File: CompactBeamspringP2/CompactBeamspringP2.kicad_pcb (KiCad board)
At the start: 2 copper layers, 162.3 x 33.2 mm, 54 parts, among them J1 BEAMSPRING CONNECTOR, J3 EXPANSION HEADER, U1 MCP4921-E, U2 LM339A, U3 74AHC595, U4 74AHC595, U5 ProMicro, U7 74AHC595

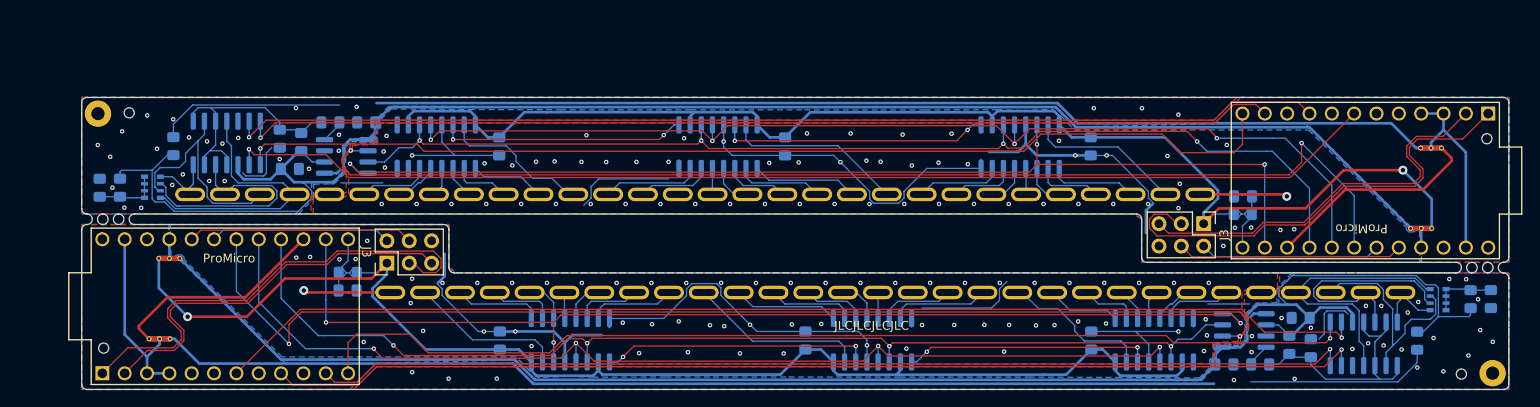
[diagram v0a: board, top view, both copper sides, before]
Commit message: More mods
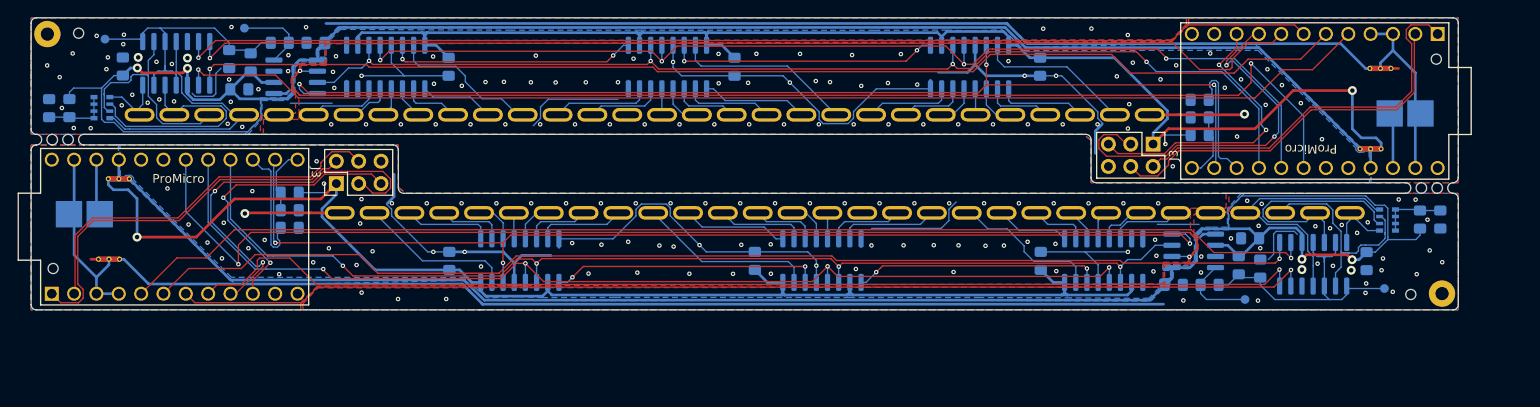
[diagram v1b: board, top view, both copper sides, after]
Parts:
- removed the C1 at (238.6, 138.5)
- removed the C1 at (141.0, 111.0)
- removed the C2 at (156.2, 135.8)
- removed the C2 at (223.4, 113.7)
- removed the C3 at (260.5, 135.8)
- removed the C3 at (119.1, 113.7)
- removed the C4 at (191.0, 135.8)
- removed the C4 at (188.7, 113.7)
- removed the C5 at (223.5, 135.8)
- removed the C5 at (156.2, 113.7)
- removed the C6 at (247.3, 133.2)
- removed the C6 at (132.4, 116.3)
- removed the H1 at (269.1, 139.5)
- removed the H1 at (110.5, 110.0)
- removed the J1 at (201.2, 130.3)
- removed the J1 at (178.4, 119.2)
- removed the J3 at (143.4, 127.0)
- removed the J3 at (236.3, 122.5)
- removed the NT1 at (116.4, 135.6)
- removed the NT1 at (263.3, 113.9)
- removed the NT2 at (117.5, 126.5)
- removed the NT2 at (262.2, 123.0)
- removed the R1 at (266.6, 131.1)
- removed the R1 at (113.1, 118.4)
- removed the R2 at (268.9, 131.1)
- removed the R2 at (110.7, 118.4)
- removed the R3 at (246.0, 136.3)
- removed the R3 at (133.7, 113.2)
- removed the R4 at (242.7, 138.5)
- removed the R4 at (137.0, 111.0)
- removed the R5 at (248.4, 136.7)
- removed the R5 at (131.2, 112.8)
- removed the R6 at (138.9, 128.1)
- removed the R6 at (240.7, 121.4)
- removed the R7 at (138.9, 130.1)
- removed the R7 at (240.7, 119.4)
- removed the REF** at (111.2, 136.7)
- removed the REF** at (265.6, 139.6)
- removed the REF** at (268.4, 112.8)
- removed the REF** at (114.1, 109.9)
- removed the RN1 at (262.9, 131.1)
- removed the RN1 at (116.7, 118.4)
- removed the U1 at (240.9, 134.6)
- removed the U1 at (138.8, 114.9)
- removed the U2 at (254.5, 136.2)
- removed the U2 at (125.2, 113.3)
- removed the U3 at (164.3, 135.8)
- removed the U3 at (215.4, 113.7)
- removed the U4 at (198.6, 135.8)
- removed the U4 at (181.0, 113.7)
- removed the U5 at (125.0, 131.9)
- removed the U5 at (254.6, 117.6)
- removed the U7 at (230.6, 135.8)
- removed the U7 at (149.0, 113.7)
- added C1: 0U1, Capacitor_SMD:C_0805_2012Metric_Pad1.15x1.40mm_HandSolder, B.Cu at (232.9, 129.5)
- added C1: 0U1, Capacitor_SMD:C_0805_2012Metric_Pad1.15x1.40mm_HandSolder, B.Cu at (135.3, 101.9)
- added C2: 0U1, Capacitor_SMD:C_0805_2012Metric_Pad1.15x1.40mm_HandSolder, B.Cu at (150.5, 126.7)
- added C2: 0U1, Capacitor_SMD:C_0805_2012Metric_Pad1.15x1.40mm_HandSolder, B.Cu at (217.7, 104.7)
- added C3: 0U1, Capacitor_SMD:C_0805_2012Metric_Pad1.15x1.40mm_HandSolder, B.Cu at (254.8, 126.8)
- added C3: 0U1, Capacitor_SMD:C_0805_2012Metric_Pad1.15x1.40mm_HandSolder, B.Cu at (113.4, 104.6)
- added C4: 0U1, Capacitor_SMD:C_0805_2012Metric_Pad1.15x1.40mm_HandSolder, B.Cu at (185.2, 126.7)
- added C4: 0U1, Capacitor_SMD:C_0805_2012Metric_Pad1.15x1.40mm_HandSolder, B.Cu at (182.9, 104.7)
- added C5: 0U1, Capacitor_SMD:C_0805_2012Metric_Pad1.15x1.40mm_HandSolder, B.Cu at (217.7, 126.7)
- added C5: 0U1, Capacitor_SMD:C_0805_2012Metric_Pad1.15x1.40mm_HandSolder, B.Cu at (150.4, 104.7)
- added C6: 0U1, Capacitor_SMD:C_0805_2012Metric_Pad1.15x1.40mm_HandSolder, B.Cu at (241.5, 124.2)
- added C6: 0U1, Capacitor_SMD:C_0805_2012Metric_Pad1.15x1.40mm_HandSolder, B.Cu at (126.6, 107.2)
- added H1: MountingHole_Pad, TH-XWhatsIt:ChassisGnd, B.Cu at (263.4, 130.4)
- added H1: MountingHole_Pad, TH-XWhatsIt:ChassisGnd, B.Cu at (104.8, 101.0)
- added J1: BEAMSPRING CONNECTOR, TH-XWhatsIt:30-pin-universal-beamspring-connector_v2, F.Cu at (195.5, 121.3)
- added J1: BEAMSPRING CONNECTOR, TH-XWhatsIt:30-pin-universal-beamspring-connector_v2, F.Cu at (172.7, 110.1)
- added J2: PadsToShort, TH-XWhatsIt:PadsToShort, B.Cu at (109.0, 118.5)
- added J2: PadsToShort, TH-XWhatsIt:PadsToShort, B.Cu at (259.1, 112.9)
- added J3: EXPANSION HEADER, Connector_PinHeader_2.54mm:PinHeader_2x03_P2.54mm_Vertical, F.Cu at (137.6, 117.9)
- added J3: EXPANSION HEADER, Connector_PinHeader_2.54mm:PinHeader_2x03_P2.54mm_Vertical, F.Cu at (230.5, 113.5)
- added NT1: Net-Tie_3, NetTie:NetTie-3_THT_Pad0.3mm, B.Cu at (110.6, 126.5)
- added NT1: Net-Tie_3, NetTie:NetTie-3_THT_Pad0.3mm, B.Cu at (257.5, 104.9)
- added NT2: Net-Tie_3, NetTie:NetTie-3_THT_Pad0.3mm, B.Cu at (111.7, 117.4)
- added NT2: Net-Tie_3, NetTie:NetTie-3_THT_Pad0.3mm, B.Cu at (256.4, 114.0)
- added R1: 4K7, Resistor_SMD:R_0805_2012Metric_Pad1.15x1.40mm_HandSolder, B.Cu at (260.8, 122.0)
- added R1: 4K7, Resistor_SMD:R_0805_2012Metric_Pad1.15x1.40mm_HandSolder, B.Cu at (107.3, 109.4)
- added R2: 1K, Resistor_SMD:R_0805_2012Metric_Pad1.15x1.40mm_HandSolder, B.Cu at (263.2, 122.0)
- added R2: 1K, Resistor_SMD:R_0805_2012Metric_Pad1.15x1.40mm_HandSolder, B.Cu at (105.0, 109.4)
- added R3: 20K, Resistor_SMD:R_0805_2012Metric_Pad1.15x1.40mm_HandSolder, B.Cu at (240.2, 127.2)
- added R3: 20K, Resistor_SMD:R_0805_2012Metric_Pad1.15x1.40mm_HandSolder, B.Cu at (127.9, 104.2)
- added R4: 20K, Resistor_SMD:R_0805_2012Metric_Pad1.15x1.40mm_HandSolder, B.Cu at (236.9, 129.5)
- added R4: 20K, Resistor_SMD:R_0805_2012Metric_Pad1.15x1.40mm_HandSolder, B.Cu at (131.2, 101.9)
- added R5: 4K7, Resistor_SMD:R_0805_2012Metric_Pad1.15x1.40mm_HandSolder, B.Cu at (242.7, 127.6)
- added R5: 4K7, Resistor_SMD:R_0805_2012Metric_Pad1.15x1.40mm_HandSolder, B.Cu at (125.5, 103.8)
- added R6: Not Mounted, Resistor_SMD:R_0805_2012Metric_Pad1.15x1.40mm_HandSolder, B.Cu at (132.3, 119.0)
- added R6: Not Mounted, Resistor_SMD:R_0805_2012Metric_Pad1.15x1.40mm_HandSolder, B.Cu at (235.8, 112.4)
- added R7: Not Mounted, Resistor_SMD:R_0805_2012Metric_Pad1.15x1.40mm_HandSolder, B.Cu at (132.3, 121.0)
- added R7: Not Mounted, Resistor_SMD:R_0805_2012Metric_Pad1.15x1.40mm_HandSolder, B.Cu at (235.8, 110.4)
- added R8: Not Mounted, Resistor_SMD:R_0805_2012Metric_Pad1.15x1.40mm_HandSolder, B.Cu at (132.3, 123.0)
- added R8: Not Mounted, Resistor_SMD:R_0805_2012Metric_Pad1.15x1.40mm_HandSolder, B.Cu at (235.8, 108.4)
- added REF**: tooling_hole, TH-XWhatsIt:tooling_hole, F.Cu at (105.5, 127.6)
- added REF**: tooling_hole, TH-XWhatsIt:tooling_hole, F.Cu at (259.8, 130.6)
- added REF**: tooling_hole, TH-XWhatsIt:tooling_hole, F.Cu at (262.7, 103.8)
- added REF**: tooling_hole, TH-XWhatsIt:tooling_hole, F.Cu at (108.3, 100.8)
- added RN1: 100K, Resistor_SMD:R_Array_Convex_4x0603, B.Cu at (257.2, 122.1)
- added RN1: 100K, Resistor_SMD:R_Array_Convex_4x0603, B.Cu at (111.0, 109.3)
- added TP1: Dac Output, TestPoint:TestPoint_Pad_D1.0mm, B.Cu at (240.9, 131.1)
- added TP1: Dac Output, TestPoint:TestPoint_Pad_D1.0mm, B.Cu at (127.2, 100.3)
- added TP2: Threshold Voltage, TestPoint:TestPoint_Pad_D1.0mm, B.Cu at (256.8, 129.9)
- added TP2: Threshold Voltage, TestPoint:TestPoint_Pad_D1.0mm, B.Cu at (111.3, 101.5)
- added U1: MCP4921-E, Package_SO:SOIC-8_3.9x4.9mm_P1.27mm, B.Cu at (235.1, 125.6)
- added U1: MCP4921-E, Package_SO:SOIC-8_3.9x4.9mm_P1.27mm, B.Cu at (133.0, 105.8)
- added U2: LM339A, Package_SO:SOIC-14_3.9x8.7mm_P1.27mm, B.Cu at (248.7, 127.1)
- added U2: LM339A, Package_SO:SOIC-14_3.9x8.7mm_P1.27mm, B.Cu at (119.4, 104.3)
- added U3: 74AHC595, Package_SO:SOIC-16_3.9x9.9mm_P1.27mm, B.Cu at (158.5, 126.7)
- added U3: 74AHC595, Package_SO:SOIC-16_3.9x9.9mm_P1.27mm, B.Cu at (209.6, 104.7)
- added U4: 74AHC595, Package_SO:SOIC-16_3.9x9.9mm_P1.27mm, B.Cu at (192.9, 126.7)
- added U4: 74AHC595, Package_SO:SOIC-16_3.9x9.9mm_P1.27mm, B.Cu at (175.3, 104.7)
- added U5: ProMicro, promicro:ProMicro, F.Cu at (119.3, 122.8)
- added U5: ProMicro, promicro:ProMicro, F.Cu at (248.9, 108.6)
- added U7: 74AHC595, Package_SO:SOIC-16_3.9x9.9mm_P1.27mm, B.Cu at (224.9, 126.7)
- added U7: 74AHC595, Package_SO:SOIC-16_3.9x9.9mm_P1.27mm, B.Cu at (143.3, 104.7)
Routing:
- net HEADER3: track 41.2 -> 89.9 mm
- net GNDD: track 267.9 -> 221.8 mm, vias 126 -> 146
- net GND: track 0.00 -> 44.3 mm
- net Net-(NT1-Pad2): track 42.9 -> 0.00 mm
- net GNDA: track 305.2 -> 262.6 mm, vias 52 -> 64
- net HEADER4: track 51.4 -> 87.2 mm
- net Net-(R8-Pad1): track 0.00 -> 30.3 mm
- net ROW1: track 239.3 -> 265.6 mm
- net HEADER2: track 90.4 -> 66.9 mm, vias 0 -> 4
- net +5VD: track 296.1 -> 317.2 mm
- net HEADER1: track 108.4 -> 87.8 mm, vias 0 -> 4
- net +5VA: track 373.7 -> 393.7 mm, vias 0 -> 4
- net ROW3: track 236.3 -> 255.7 mm
- net RST: track 0.00 -> 12.7 mm
- net Net-(R4-Pad2): track 5.33 -> 18.0 mm
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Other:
- outline, holes or cut-outs redrawn
- board text added: "Compact-Beamspring Rev1.2"
- board text added: "DAC"
- board text added: "Threshold"
- board text added: "Voltage"
- board text added: "Vout"
- board text removed: "Compact-Beamspring Rev1.1"
- board text removed: "JLCJLCJLCJLC"
